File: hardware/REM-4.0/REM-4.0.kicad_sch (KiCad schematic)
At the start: 33 parts, among them J1 PinHeader_2.54mm 02x04 Horizo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, J2 PinHeader_2.54mm 02x05 Horizo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, Q1 IRLB3034PbF, U1 NE555P

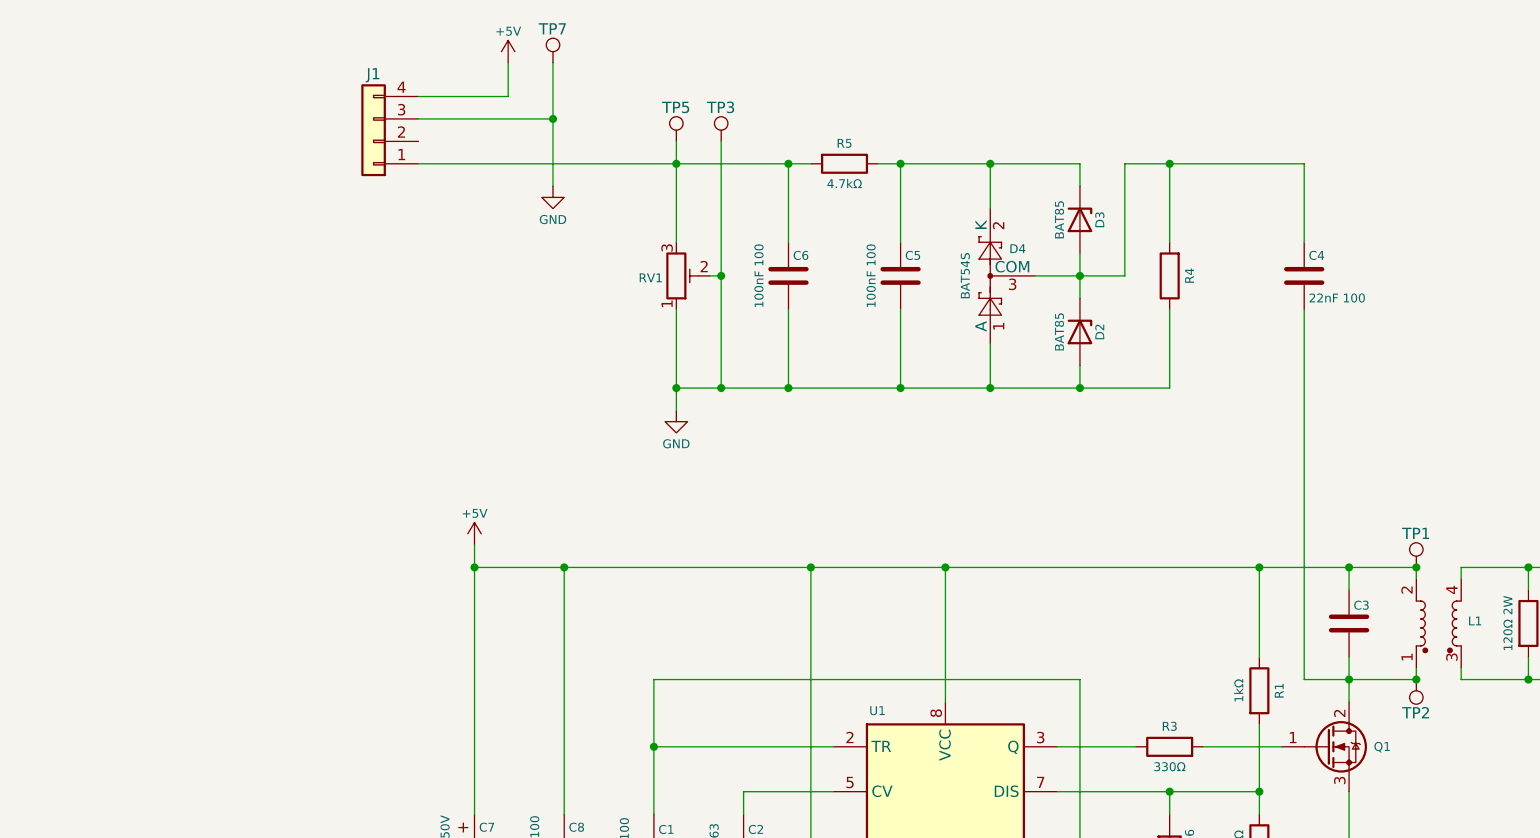
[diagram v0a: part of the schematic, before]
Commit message: modified:   .DS_Store 	modified:   Ferrite Transformer Calculation.xlsx 	new file:   archive/REM - Vsense.xlsx 	new file:   hardware/INA-1.0/#auto_saved_files# 	new file:   hardware/INA-1.0/INA-1.0-backups/INA-1.0-2026-04-10_134714.zip 	new file:   hardware/INA-1.0/INA-1.0-backups/INA-1.0-2026-04-10_141544.zip 	new file:   hardware/INA-1.0/INA-1.0-backups/INA-1.0-2026-04-10_154242.zip 	new file:   hardware/INA-1.0/INA-1.0-backups/INA-1.0-2026-04-10_161020.zip 	new file:   hardware/INA-1.0/INA-1.0-backups/INA-1.0-2026-04-10_163134.zip 	new file:   hardware/INA-1.0/INA-1.0-backups/INA-1.0-2026-04-12_233203.zip 	new file:   hardware/INA-1.0/INA-1.0-backups/INA-1.0-2026-04-12_234518.zip 	new file:   hardware/INA-1.0/INA-1.0-backups/INA-1.0-2026-04-13_105232.zip 	new file:   hardware/INA-1.0/INA-1.0-backups/INA-1.0-2026-04-13_105845.zip 	new file:   hardware/INA-1.0/INA-1.0-backups/INA-1.0-2026-04-13_110346.zip 	new file:   hardware/INA-1.0/INA-1.0-backups/INA-1.0-2026-04-13_112014.zip 	new file:   hardware/INA-1.0/INA-1.0-backups/INA-1.0-2026-04-13_112658.zip 	new file:   hardware/INA-1.0/INA-1.0-backups/INA-1.0-2026-04-13_114201.zip 	new file:   hardware/INA-1.0/INA-1.0.kicad_pcb 	new file:   hardware/INA-1.0/INA-1.0.kicad_prl 	new file:   hardware/INA-1.0/INA-1.0.kicad_pro 	new file:   hardware/INA-1.0/INA-1.0.kicad_sch 	new file:   hardware/INA-1.0/_autosave-INA-1.0.kicad_pcb 	new file:   hardware/INA-1.0/_autosave-INA-1.0.kicad_sch 	new file:   hardware/INA-1.0/fabrication-outputs/INA-1.0-F_Cu.dxf 	new file:   hardware/INA-1.0/fabrication-outputs/INA-1.0-F_Mask.dxf 	new file:   hardware/INA-1.0/fabrication-outputs/INA-1.0-NPTH-drl_map.dxf 	new file:   hardware/INA-1.0/fabrication-outputs/INA-1.0-PTH-drl_map.dxf 	new file:   hardware/INA-1.0/fabrication-outputs/TRACE.dxf 	new file:   hardware/INA-1.0/fp-info-cache 	renamed:    hardware/REM-4.0/~REM-4.0.kicad_pcb.lck -> hardware/INA-1.0/~INA-1.0.kicad_sch.lck 	new file:   hardware/INA-1.0/~_autosave-INA-1.0.kicad_pcb.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
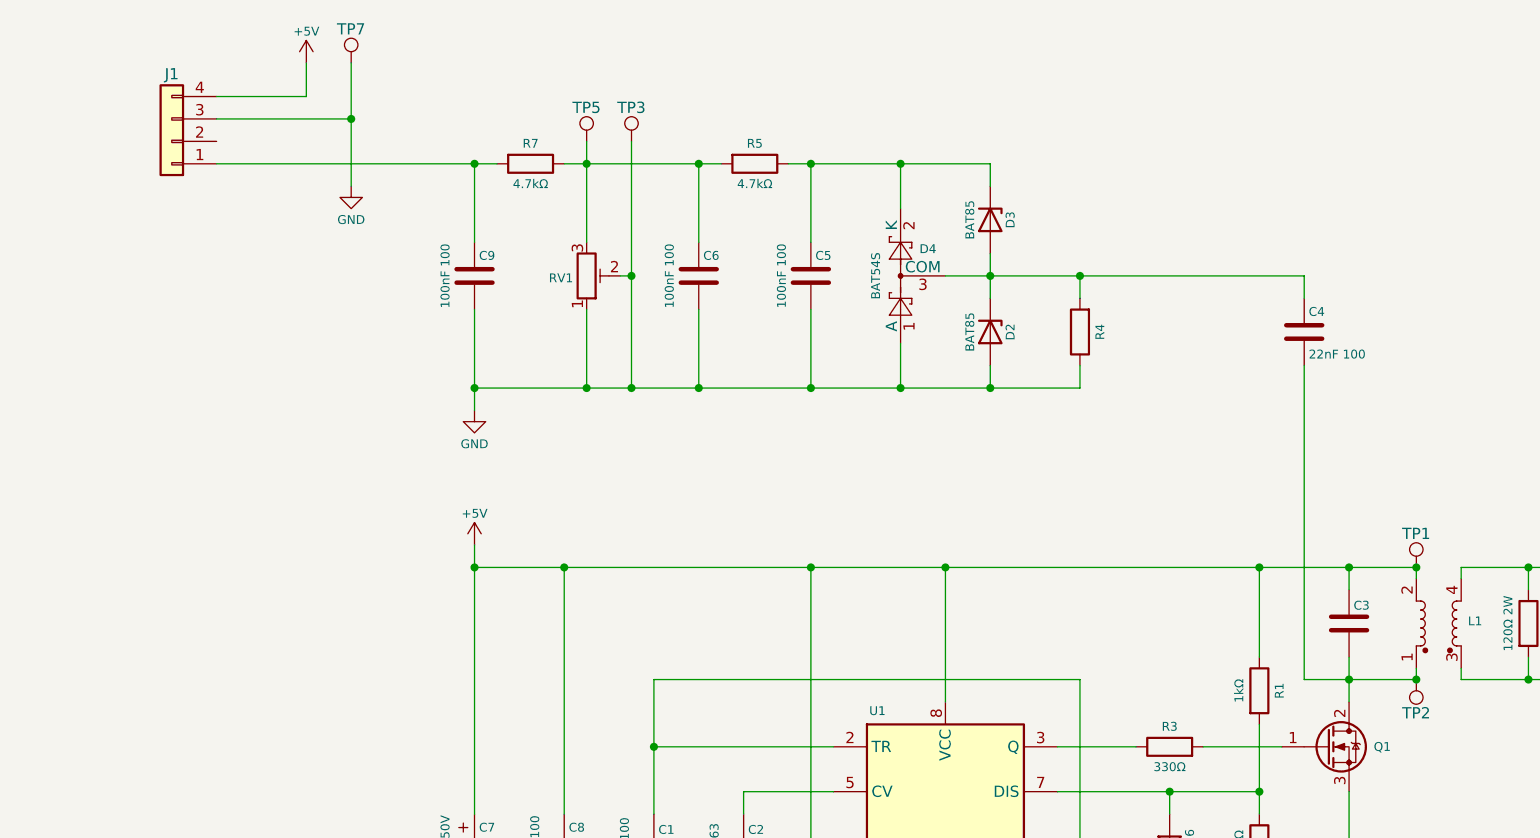
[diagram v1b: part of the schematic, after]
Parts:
- added C9: 100nF 100, Capacitor_THT:C_Rect_L7.0mm_W3.5mm_P5.00mm, symbol Device:C
- added R7: 4.7kΩ, Resistor_THT:R_Axial_DIN0204_L3.6mm_D1.6mm_P7.62mm_Horizontal, symbol Device:R
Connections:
- net GND: now also C9.2
- net at C6.1, R5.2, RV1.3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: now also R7.1; no longer J1.1 (Pin_1)
- new net: C9.1, J1.1 (Pin_1), R7.2
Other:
- moved on the sheet: C4, C5, C6, D2, D3, D4, J1, R4, R5, RV1, TP3, TP5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
